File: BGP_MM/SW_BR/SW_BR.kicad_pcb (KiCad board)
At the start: 2 copper layers, 12 x 13 mm, 2 parts, among them P1 CONN_01X03, P2 CONN_01X02

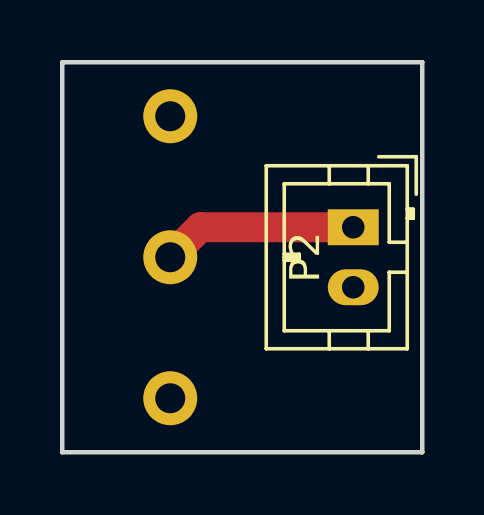
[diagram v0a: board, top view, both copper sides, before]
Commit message: MM Gerbers, BASS pot fixup
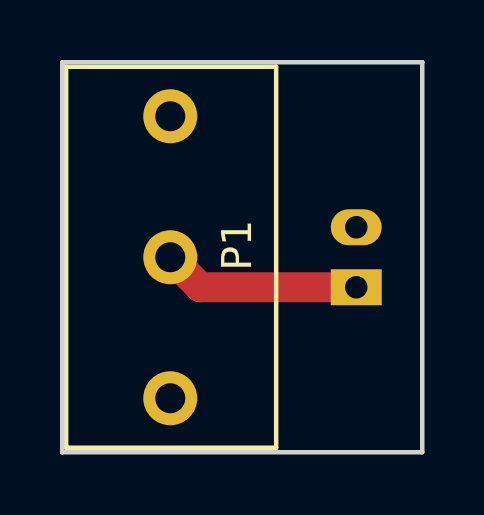
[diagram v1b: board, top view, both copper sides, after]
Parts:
- P1: moved to F.Cu
- P2: moved to B.Cu
- moved P1 9.40 mm to (141.6, 111.2), turned to 270 degrees
- moved P2 2.00 mm to (147.8, 107.5), turned to 90 degrees
